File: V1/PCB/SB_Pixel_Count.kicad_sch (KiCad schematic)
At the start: 17 parts, among them J2 String1, J3 OLED, SW1 Test, U1 74AHCT1G125, U3 AMS1117-5.0, U4 INA219BxD, U5 RP2040-Tiny

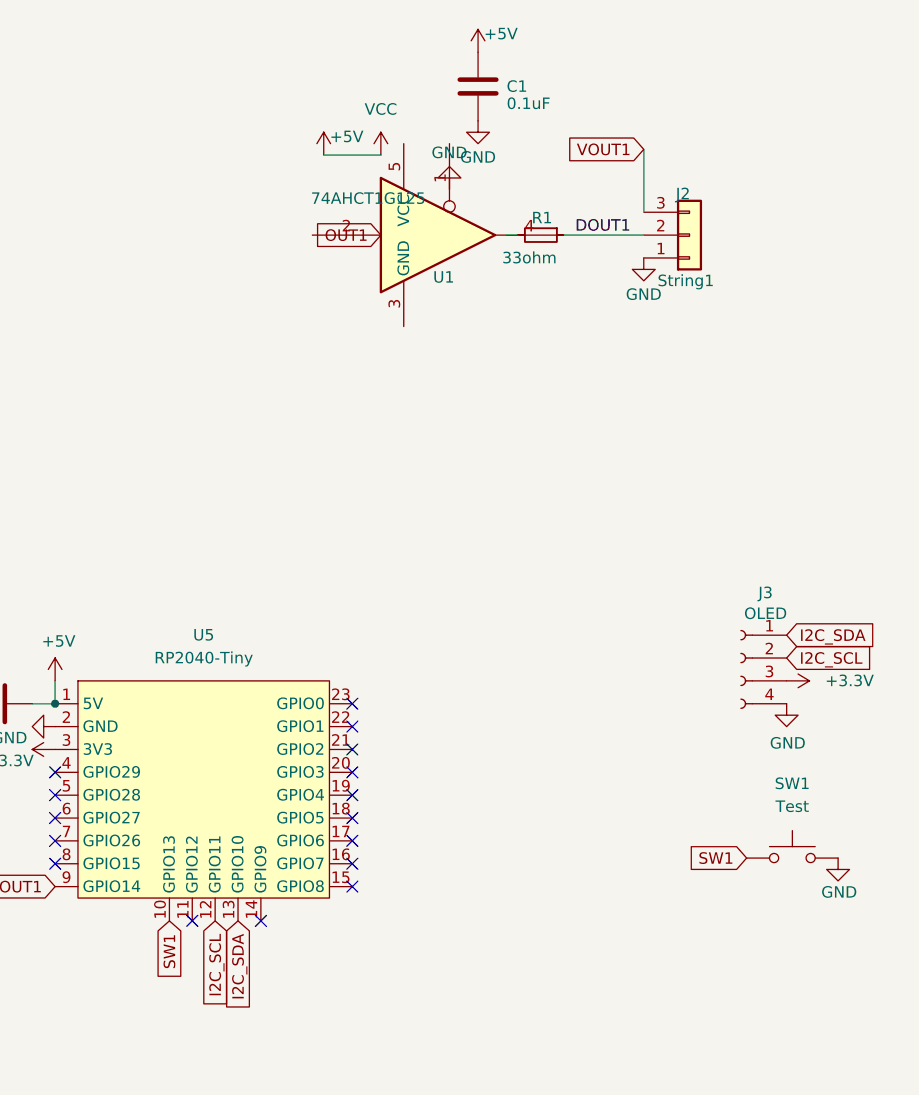
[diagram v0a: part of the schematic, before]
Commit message: v1 fixes
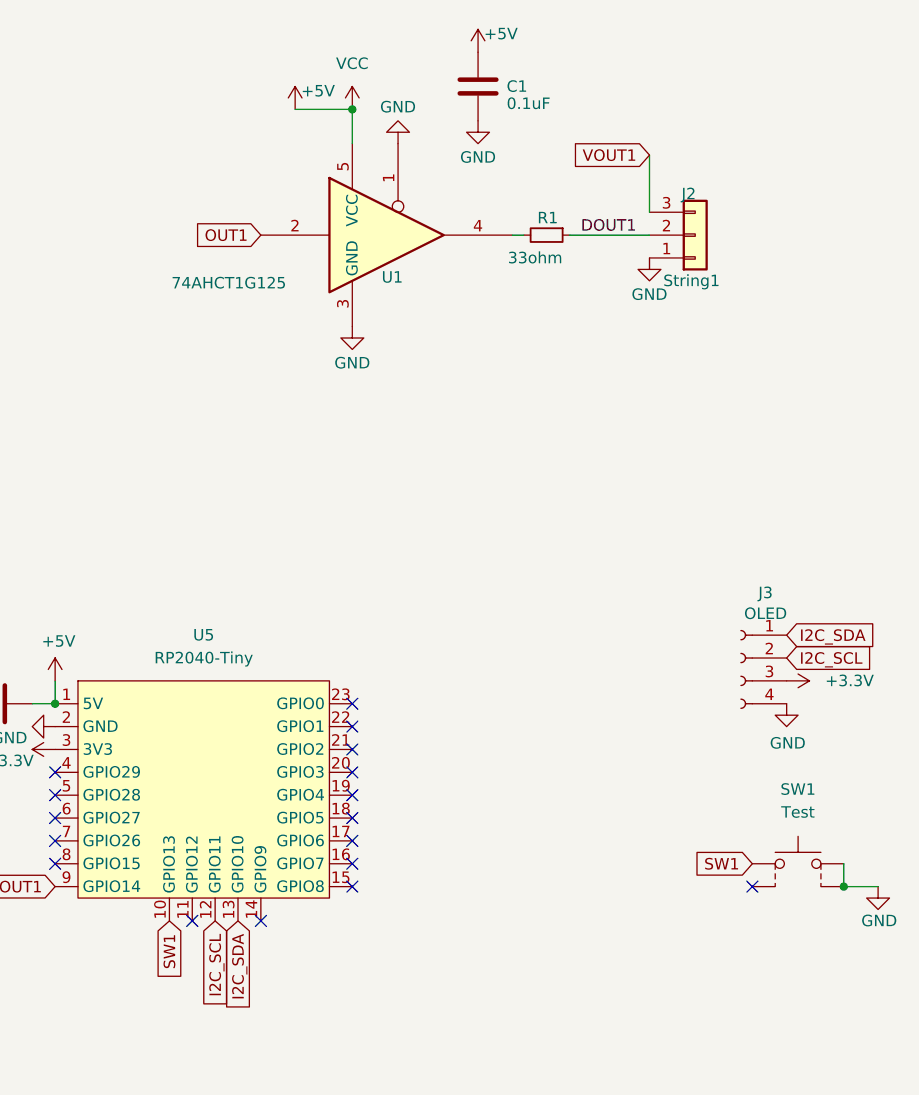
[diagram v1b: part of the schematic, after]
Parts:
- SW1: footprint Button_Switch_SMD:SW_Push_1P1T_NO_6x6mm_H9.5mm -> Scotts:SW_Push_1P1T_NO_6x6mm_H9.5mm; symbol Switch:SW_Push -> Scotts:SW_PUSH_6mm
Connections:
- net +5V: now also U1.5 (VCC)
- net DOUT1: no longer U1.4
- net GND: now also SW1.4, U1.1, U1.3 (GND)
- net OUT1: now also U1.2
- net at R1.2: now also U1.4
- no-connect marks 17 -> 18
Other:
- moved on the sheet: J2, R1, U1
